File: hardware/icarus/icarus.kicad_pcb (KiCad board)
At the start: 4 copper layers, 37.1 x 43.3 mm, 43 parts, among them J1 BAT, J2 IO, J3 I2C_EX, J4 UART, P1 USB_C_Plug_USB2.0, Q1 DMG2305, SW1 USER, SW2 RST, U1 AMS1117-3.3, U2 BMM150, U4 MPU-6050, U6 BMP388, U7 ESP32-C3-MINI-1

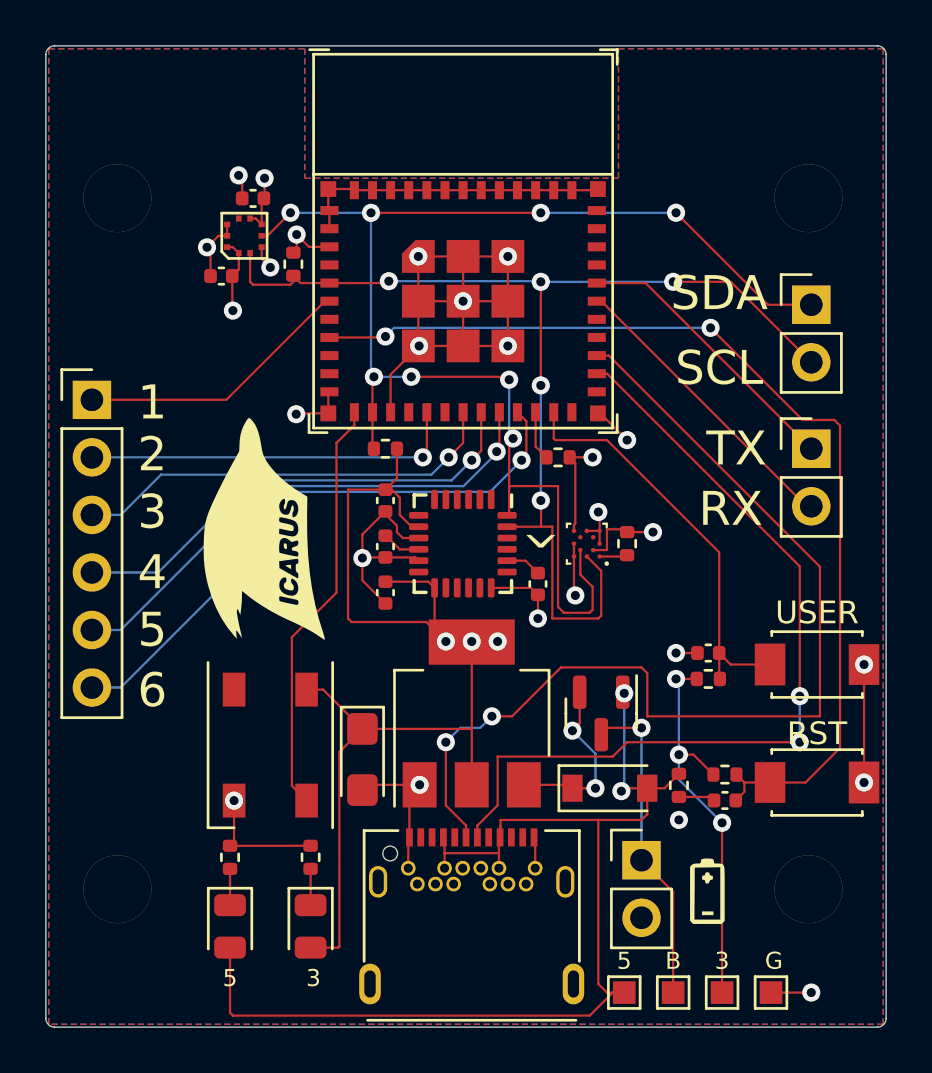
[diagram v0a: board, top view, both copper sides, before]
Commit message: Rev D.2
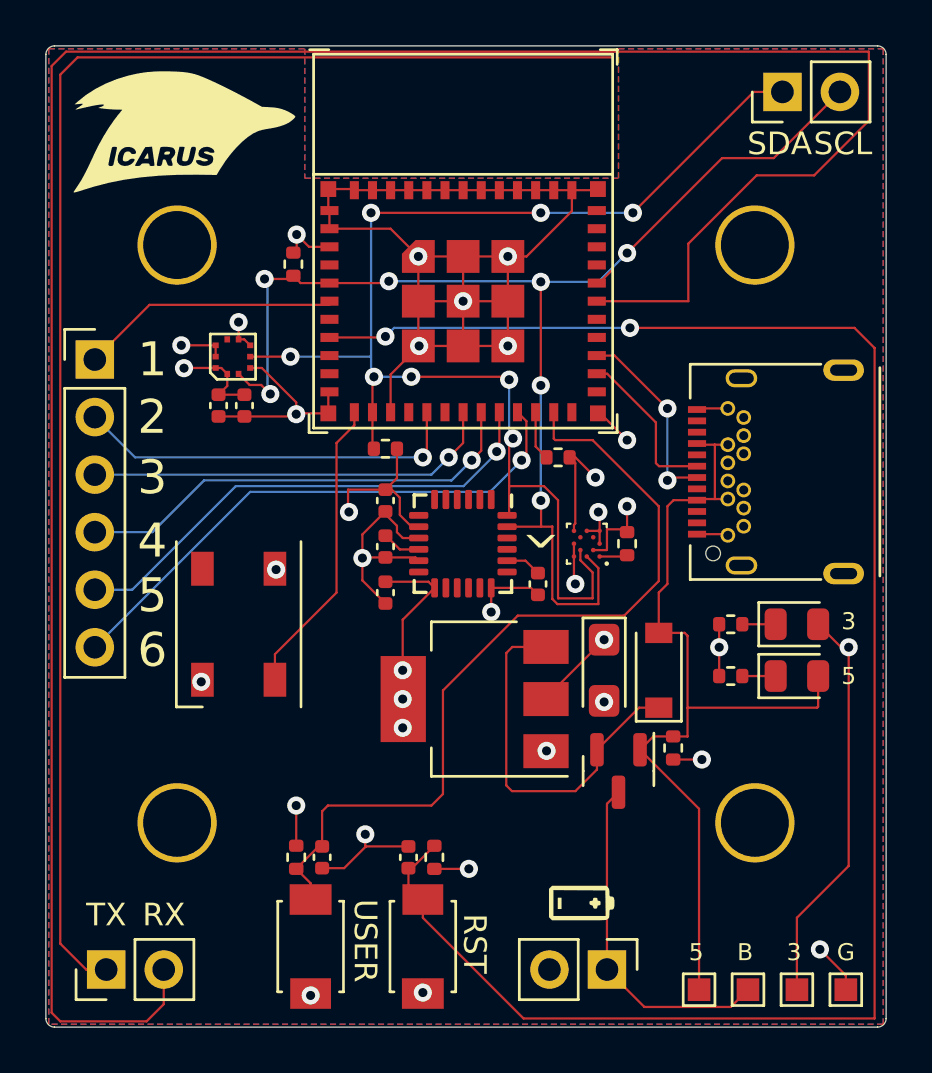
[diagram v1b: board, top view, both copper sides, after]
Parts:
- removed the REF** at (149.1, 71.5)
- added REF**: mounting_holes_25.5mm, drone:mounting_holes_25.5mm, F.Cu at (149.2, 71.1)
- moved J4 38.7 mm to (133.3, 90.3), turned to 90 degrees
- moved D2 27.4 mm to (163.8, 77.3), turned to 0 degrees
- moved P1 26.0 mm to (164.5, 68.3), turned to 90 degrees
- moved SW1 25.6 mm to (142.4, 89.3), turned to 90 degrees
- moved D3 25.3 mm to (163.8, 75.1), turned to 0 degrees
- moved R4 23.5 mm to (160.9, 77.3), turned to 180 degrees
- moved R5 21.2 mm to (160.9, 75.1), turned to 180 degrees
- moved R12 19.8 mm to (141.7, 85.3), turned to -90 degrees
- moved C10 19.3 mm to (142.9, 85.3), turned to -90 degrees
- moved SW2 18.8 mm to (147.3, 89.3), turned to -90 degrees
- moved G*** 17.9 mm to (136.8, 53.3), turned to 0 degrees
- moved C9 14.2 mm to (146.7, 85.3), turned to 90 degrees
- moved R11 13.3 mm to (147.8, 85.3), turned to 90 degrees
- moved C1 11.4 mm to (155.3, 77.1)
- moved J3 9.48 mm to (163.2, 51.6), turned to 90 degrees
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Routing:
- net Net-(J4-Pad2): track 13.2 -> 104.9 mm
- net Net-(J4-Pad1): track 12.5 -> 75.9 mm
- net /usb_dp: track 44.8 -> 8.62 mm
- net /nreset: track 45.0 -> 80.0 mm
- net /usb_dm: track 37.8 -> 7.17 mm, vias 2 -> 0
- net +3V3: track 81.2 -> 55.0 mm, vias 11 -> 14
- net /user_btn: track 18.6 -> 36.8 mm
- net VBUS: track 50.3 -> 39.2 mm, vias 2 -> 0
- net Net-(D1-Pad1): track 8.02 -> 16.6 mm, vias 2 -> 0
- net /scl: track 50.0 -> 56.5 mm, vias 5 -> 7
- net Net-(D4-Pad4): track 18.6 -> 13.3 mm
- net GND: track 90.5 -> 92.7 mm
- net /sda: track 61.1 -> 59.0 mm
- net /io6: track 26.7 -> 24.6 mm
- net +BATT: track 14.2 -> 15.3 mm, vias 1 -> 0
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- added copper zone on F.Cu, net (none)
- removed copper zone on In1.Cu, net +BATT
- removed copper zone on F.Cu, net GND
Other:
- board text added: "icarus :: Rev D.2 nnarain"
- board text removed: "icarus :: Rev D nnarain"
